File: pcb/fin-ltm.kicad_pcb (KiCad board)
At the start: 2 copper layers, 112.5 x 109.8 mm, 167 parts, among them J1 Connector, USB-TYPE-C-16P, J2 Test Connector, Q1 MMBT3904, Q2 HL3415A, U1 ESP32-C3FH4, U2 RT9080, U3 SN74LV1T34DBV, X1 40MHz, 15pF

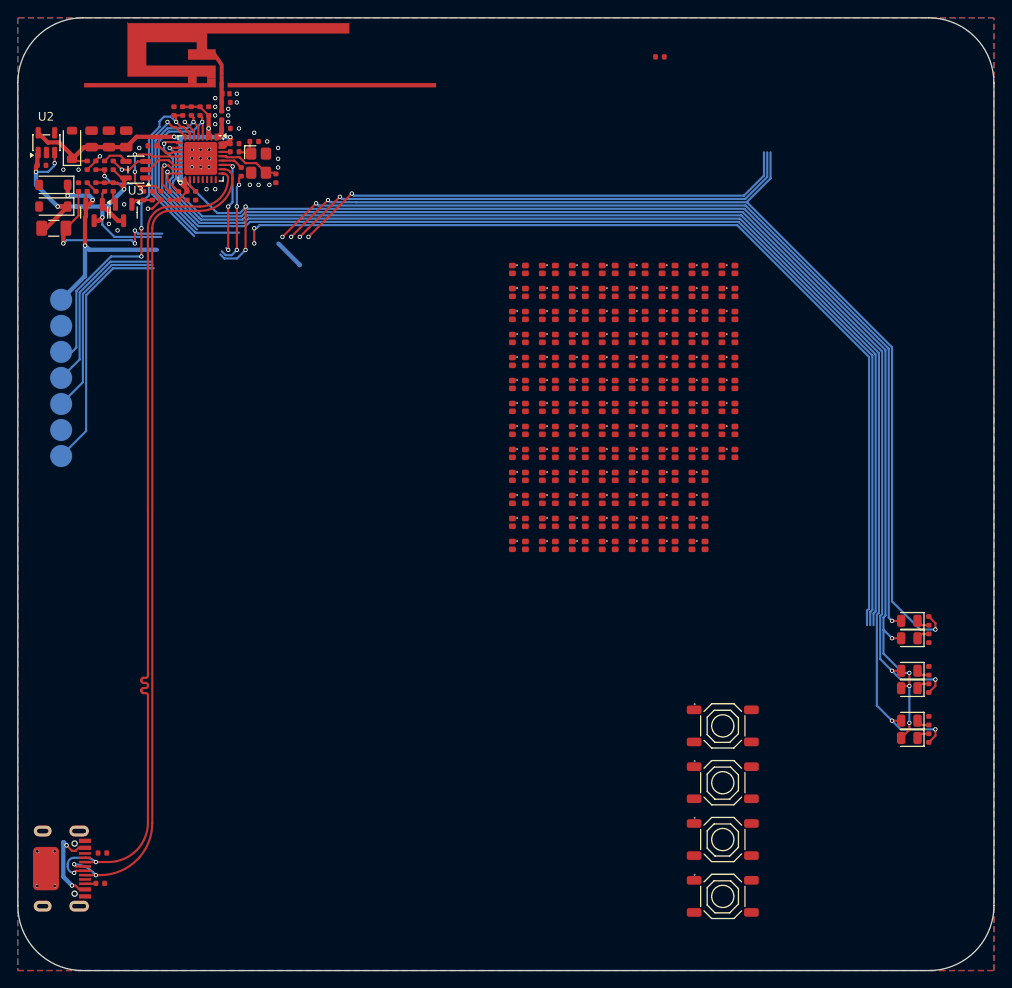
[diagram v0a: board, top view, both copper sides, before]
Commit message: pcb 2
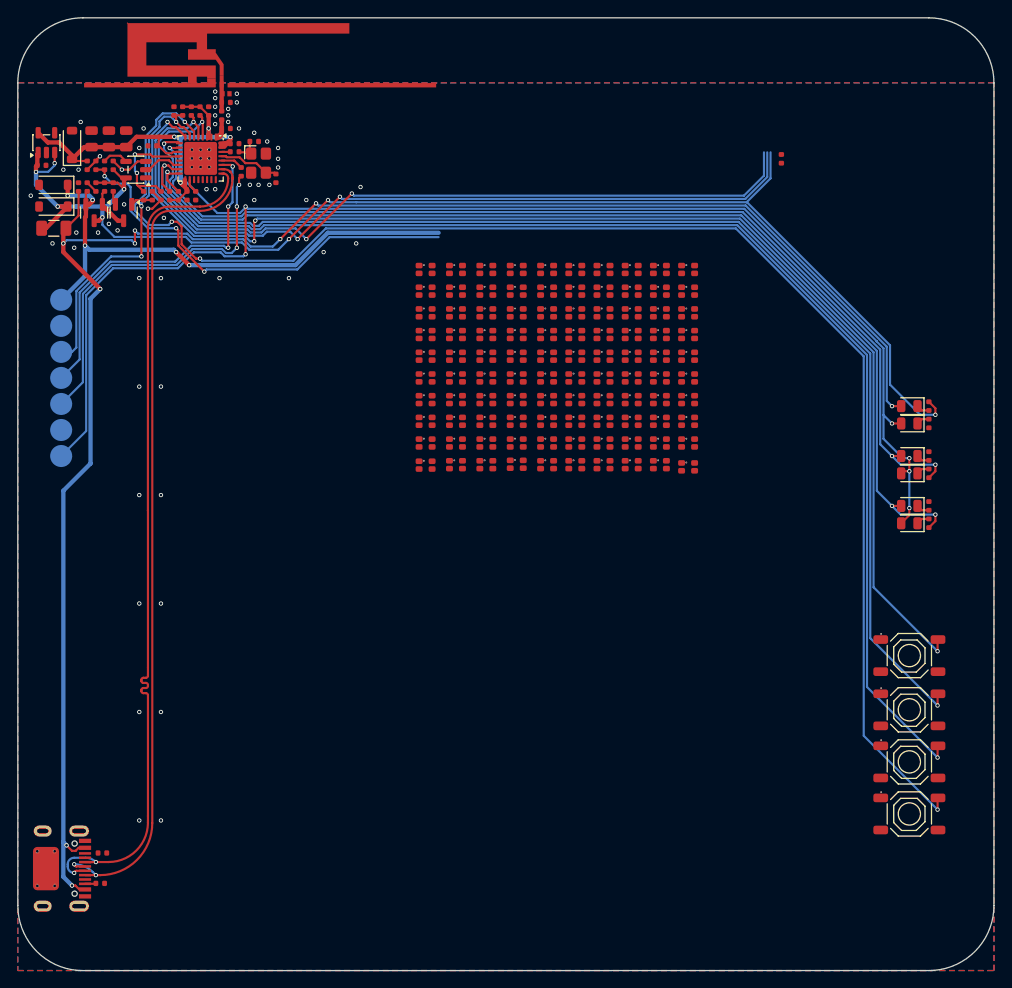
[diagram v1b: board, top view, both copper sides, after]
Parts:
- moved D191 31.8 mm to (94.8, 46.5)
- moved S3 30.2 mm to (120.2, 91.0)
- moved D152 29.6 mm to (81.8, 49.0)
- moved D151 29.4 mm to (81.8, 46.5)
- moved D113 27.8 mm to (68.0, 51.5)
- moved D112 27.6 mm to (68.0, 49.0)
- moved D111 27.5 mm to (68.0, 46.5)
- moved D140 24.8 mm to (75.0, 69.0)
- moved D1 24.8 mm to (120.2, 62.2)
- moved D10 24.8 mm to (120.2, 73.8)
- moved D5 24.8 mm to (120.2, 64.2)
- moved D7 24.8 mm to (120.2, 70.0)
- moved D8 24.8 mm to (120.2, 68.0)
- moved D9 24.8 mm to (120.2, 75.8)
- moved R12 24.8 mm to (122.5, 70.0)
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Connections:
- R16 pad 2: /BRIGHTNESS_UP_BUTTON -> /BRIGHTNESS_DOWN_BUTTON
- R17 pad 2: /BRIGHTNESS_DOWN_BUTTON -> /BRIGHTNESS_UP_BUTTON
- U1 pad 15: /BRIGHTNESS_UP_BUTTON -> /BRIGHTNESS_DOWN_BUTTON
- U1 pad 16: /BRIGHTNESS_DOWN_BUTTON -> /BRIGHTNESS_UP_BUTTON
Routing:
- net /MODE_BUTTON: track 2.19 -> 170.4 mm, vias 1 -> 4
- net Net-(C1-Pad2): track 141.2 -> 203.9 mm, vias 8 -> 9
- net /Leds/LED_DATA_5V: track 5.33 -> 49.1 mm, vias 1 -> 3
- net +5V: track 31.2 -> 62.4 mm, vias 3 -> 5
- net /SERVER_LED: track 149.1 -> 124.1 mm
- net /WIFI_LED: track 141.8 -> 116.9 mm
- net /BRIGHTNESS_DOWN_BUTTON: track 127.6 -> 148.9 mm, vias 1 -> 2
- net +3V3: track 226.8 -> 210.5 mm
- net /POWER_BUTTON: track 128.7 -> 144.9 mm, vias 3 -> 4
- net /DISPLAY_SDA: track 78.8 -> 92.6 mm
- net /BRIGHTNESS_UP_BUTTON: track 129.6 -> 140.8 mm, vias 1 -> 2
- net /MCU_RX: track 31.9 -> 41.1 mm
- net VBUS: track 164.5 -> 156.0 mm
- net /MCU_TX: track 34.0 -> 42.5 mm
- net /DISPLAY_SCL: track 85.5 -> 93.2 mm
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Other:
- board text added: "OLED here?"
- board text added: "Reroute 5V and LED_DATA traces if needed"
